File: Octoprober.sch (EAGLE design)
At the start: 98 parts, among them J1 10118193-0001LF, P1 TC33X-1, SW1 EVQ-Q2203W, SW2 EVQ-Q2203W, SW3 EVQ-Q2203W, SW4 EVQ-Q2203W, SW5 EVQ-Q2203W, U1 P8X32A-M44, U10 MAX31855KASA+, U11 MAX31855KASA+, U12 MAX31855KASA+, U13 MAX31855KASA+, U14 MAX31855KASA+, U15 PMV22EN,215, U16 PMV22EN,215, U17 PMV160UP,215, U18 AD7999YRJZ-1500RL7, U2 CAT24C512WI-GT3, U3 ADP3338AKCZ-3.3-RL, U5 BQ24075RGTT, U6 74HC2G04GV,125, U7 MAX31855KASA+, U8 MAX31855KASA+, U9 MAX31855KASA+, X1 ATS060CSM-1

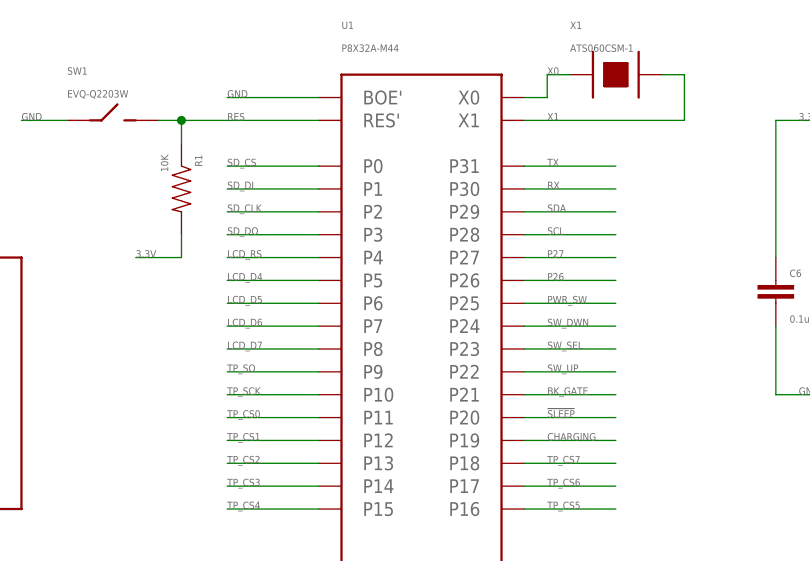
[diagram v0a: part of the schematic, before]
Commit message: Worked on the layout some more.
Still need lots of work and connectors.
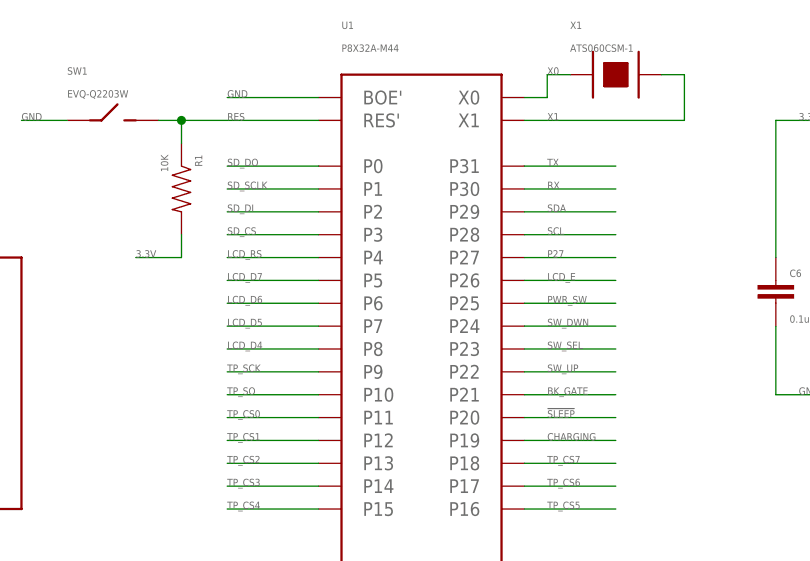
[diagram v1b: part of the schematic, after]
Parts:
- U1: device PP_DigitalIC:P8X32A_PROPELLERLQFP/QFN-44 -> PP_DigitalIC:P8X32A_PROPELLERQFN-44
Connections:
- removed net P26: U1.P26
- removed net SD_CLK: U1.P2
- net LCD_D4: now also U1.P8; no longer U1.P5
- net LCD_D5: now also U1.P7; no longer U1.P6
- net LCD_D6: now also U1.P6; no longer U1.P7
- net LCD_D7: now also U1.P5; no longer U1.P8
- net LCD_E: now also U1.P26
- net SD_CS: now also U1.P3; no longer U1.P0
- net SD_DI: now also U1.P2; no longer U1.P1
- net SD_DO: now also U1.P0; no longer U1.P3
- net SD_SCLK: now also U1.P1
- net TP_SCK: now also U1.P9; no longer U1.P10
- net TP_SO: now also U1.P10; no longer U1.P9
